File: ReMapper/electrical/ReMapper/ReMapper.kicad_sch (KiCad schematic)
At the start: 7 parts, among them SW1 PU Button, U1 ESP32-S3-WROOM-1-N8R8, U2 SC0914_13_

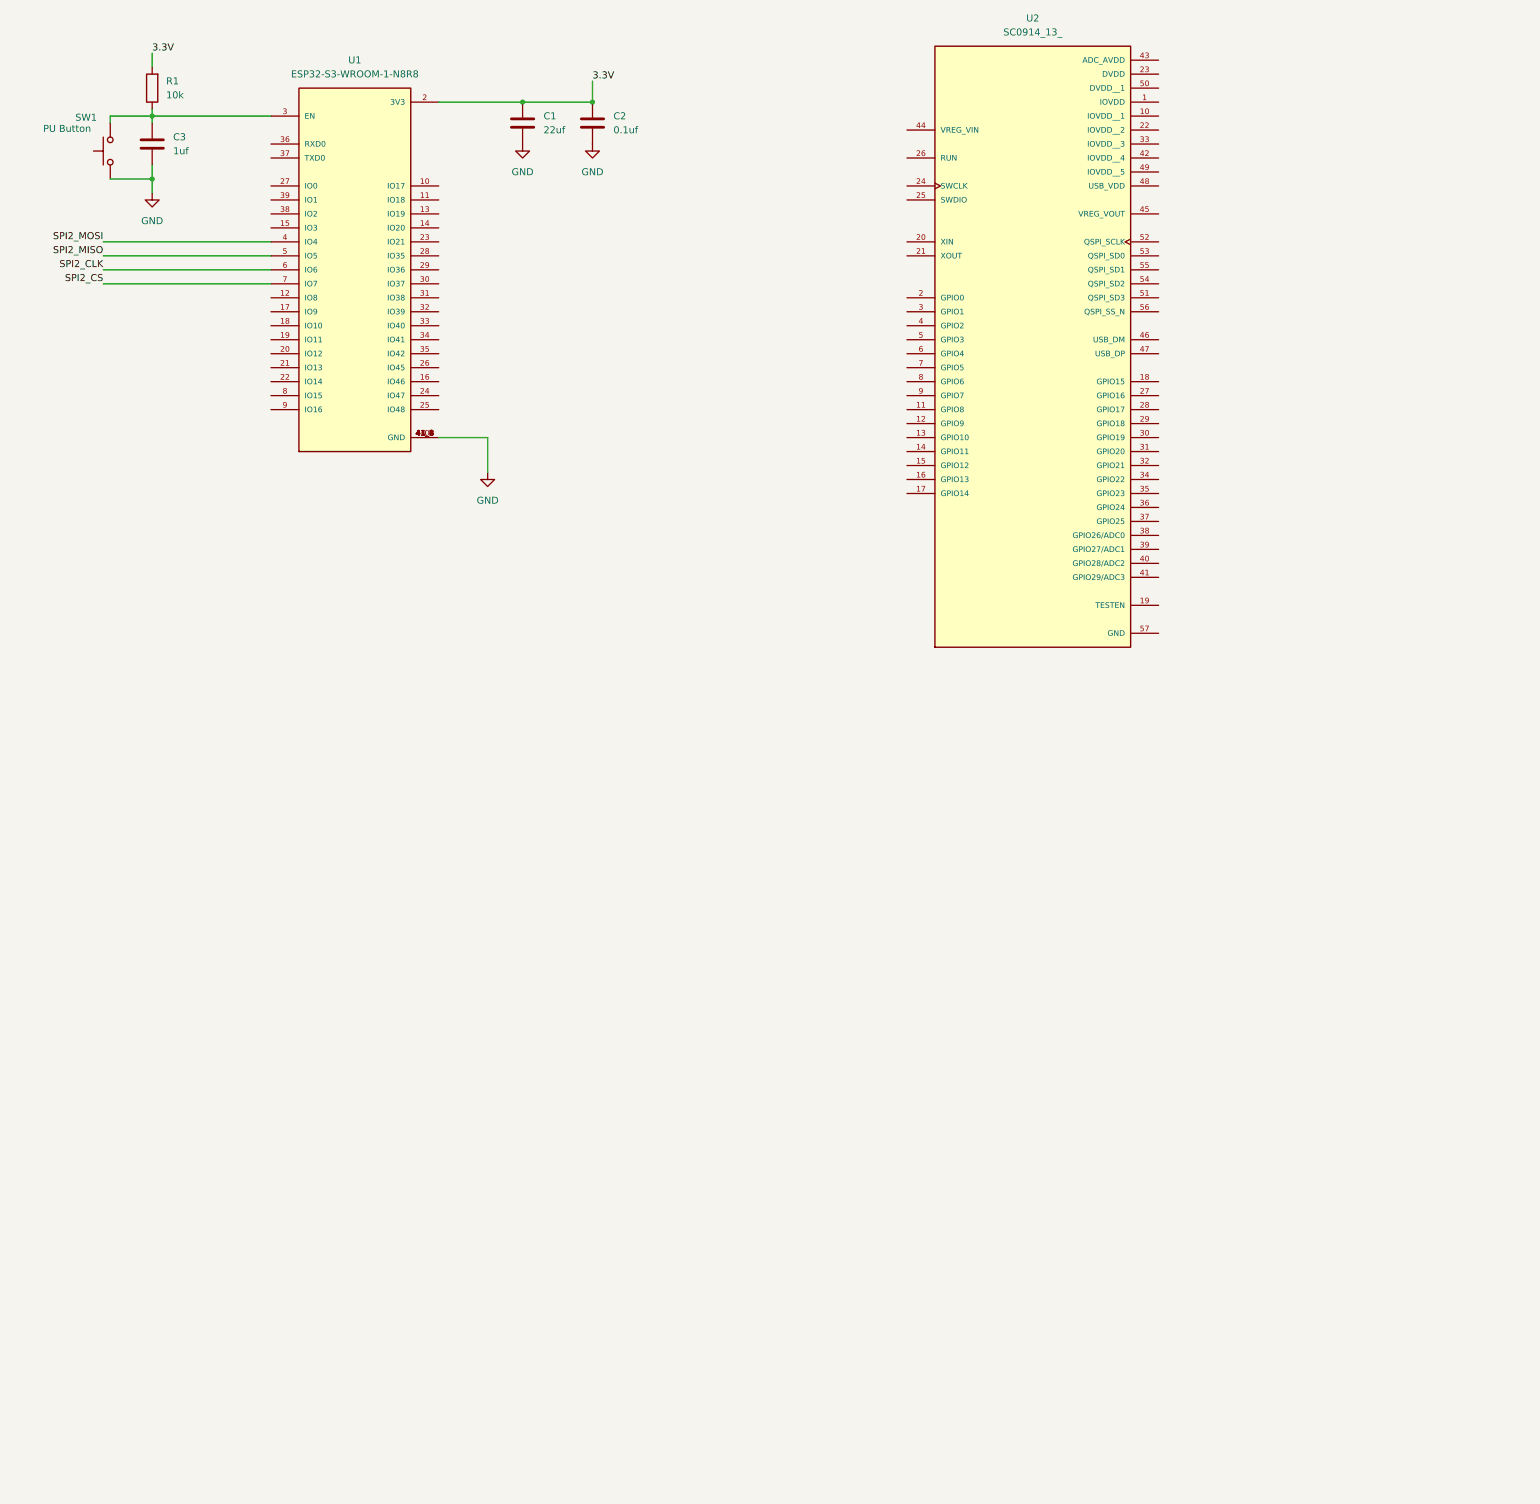
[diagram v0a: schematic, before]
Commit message: more work on schematic
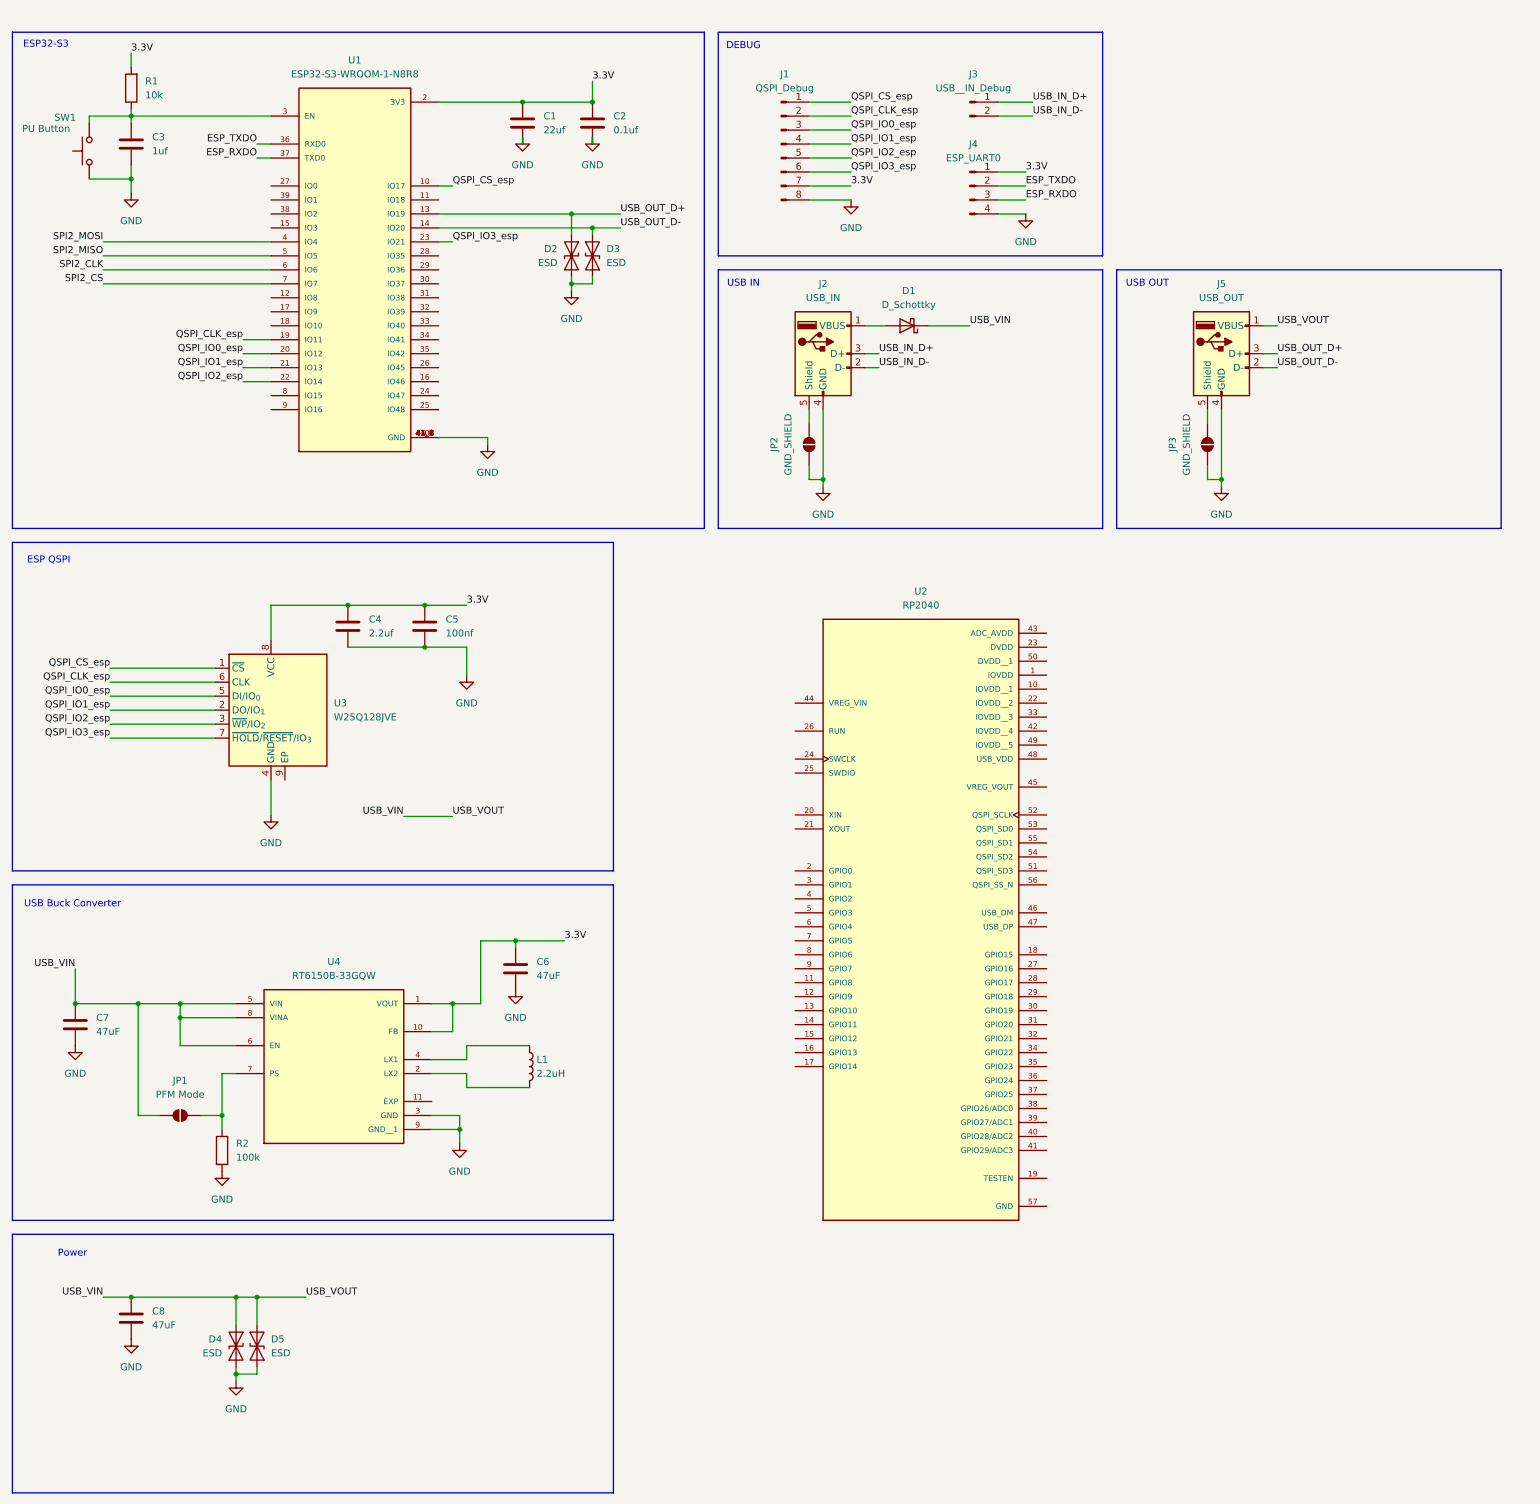
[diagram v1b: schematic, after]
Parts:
- added C4: 2.2uf, symbol Device:C
- added C5: 100nf, symbol Device:C
- added C6, C7, C8: 47uF, symbol Device:C
- added D1: D_Schottky, symbol Device:D_Schottky
- added D2, D3, D4, D5: ESD, Diode_SMD:D_SOD-523, symbol Diode:ESD9B5.0ST5G
- added J1: QSPI_Debug, Connector_PinHeader_1.00mm:PinHeader_1x08_P1.00mm_Vertical, symbol Connector:Conn_01x08_Pin
- added J2: USB_IN, footprints:USBA_Female, symbol Connector:USB_A
- added J3: USB__IN_Debug, Connector_PinHeader_1.00mm:PinHeader_1x02_P1.00mm_Vertical, symbol Connector:Conn_01x02_Pin
- added J4: ESP_UART0, Connector_PinHeader_1.00mm:PinHeader_1x04_P1.00mm_Vertical, symbol Connector:Conn_01x04_Pin
- added J5: USB_OUT, footprints:USBA_Female, symbol Connector:USB_A
- added JP1: PFM Mode, Jumper:SolderJumper-2_P1.3mm_Open_Pad1.0x1.5mm, symbol Jumper:SolderJumper_2_Open
- added JP2, JP3: GND_SHIELD, Jumper:SolderJumper-2_P1.3mm_Open_Pad1.0x1.5mm, symbol Jumper:SolderJumper_2_Open
- added L1: 2.2uH, symbol Device:L
- added R2: 100k, symbol Device:R
- added U3: W25Q128JVE, Package_SON:WSON-8-1EP_8x6mm_P1.27mm_EP3.4x4.3mm, symbol Memory_Flash:W25Q128JVE
- added U4: RT6150B-33GQW, footprints:RT6150B-33GQW, symbol RT6150B-33GQW:RT6150B-33GQW
- U2: value SC0914_13_ -> RP2040
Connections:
- net 3.3V: now also C4.1, C5.1, C6.1, J1.7 (Pin_7), J4.1 (Pin_1), U3.8 (VCC), U4.1 (VOUT), U4.10 (FB)
- net GND: now also C4.2, C5.2, C6.2, C7.2, C8.2, D2.2 (A2), D3.1 (A1), D4.2 (A2), D5.1 (A1), J1.8 (Pin_8), J2.4 (GND), J4.4 (Pin_4), J5.4 (GND), JP2.2 (B), JP3.2 (B), R2.2, U3.4 (GND), U4.3 (GND), U4.9 (GND__1)
- net QSPI_CS_esp: now reaches U1.10 (IO17)
- net QSPI_CS_esp: now also J1.1 (Pin_1), U3.1 (~{CS})
- net USB_OUT_D+: now reaches U1.13 (IO19)
- net USB_OUT_D+: now also D2.1 (A1), J5.3 (D+)
- net USB_OUT_D-: now reaches U1.14 (IO20)
- net USB_OUT_D-: now also D3.2 (A2), J5.2 (D-)
- net QSPI_CLK_esp: now reaches U1.19 (IO11)
- net QSPI_CLK_esp: now also J1.2 (Pin_2), U3.6 (CLK)
- net QSPI_IO0_esp: now reaches U1.20 (IO12)
- net QSPI_IO0_esp: now also J1.3 (Pin_3), U3.5 (DI/IO_{0})
- net QSPI_IO1_esp: now reaches U1.21 (IO13)
- net QSPI_IO1_esp: now also J1.4 (Pin_4), U3.2 (DO/IO_{1})
- net QSPI_IO2_esp: now reaches U1.22 (IO14)
- net QSPI_IO2_esp: now also J1.5 (Pin_5), U3.3 (~{WP}/IO_{2})
- net QSPI_IO3_esp: now reaches U1.23 (IO21)
- net QSPI_IO3_esp: now also J1.6 (Pin_6), U3.7 (~{HOLD}/~{RESET}/IO_{3})
- net ESP_TXDO: now reaches U1.36 (RXD0)
- net ESP_TXDO: now also J4.2 (Pin_2)
- net ESP_RXDO: now reaches U1.37 (TXD0)
- net ESP_RXDO: now also J4.3 (Pin_3)
- new net: J5.5 (Shield), JP3.1 (A)
- new net: J2.5 (Shield), JP2.1 (A)
- new net: JP1.1 (A), R2.1, U4.7 (PS)
- new net: D1.2 (A), J2.1 (VBUS)
- new net: L1.1, U4.4 (LX1)
- new net: L1.2, U4.2 (LX2)
- new net USB_IN_D+: J2.3 (D+), J3.1 (Pin_1)
- new net USB_IN_D-: J2.2 (D-), J3.2 (Pin_2)
- new net USB_VIN: C7.1, C8.1, D1.1 (K), D4.1 (A1), D5.2 (A2), J5.1 (VBUS), JP1.2 (B), U4.5 (VIN), U4.6 (EN), U4.8 (VINA)
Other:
- note added: "DEBUG"
- note added: "ESP QSPI"
- note added: "ESP32-S3"
- note added: "Power"
- note added: "USB Buck Converter"
- note added: "USB IN"
- note added: "USB OUT"
- moved on the sheet: C3, R1, SW1, U2

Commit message: first draft schematic
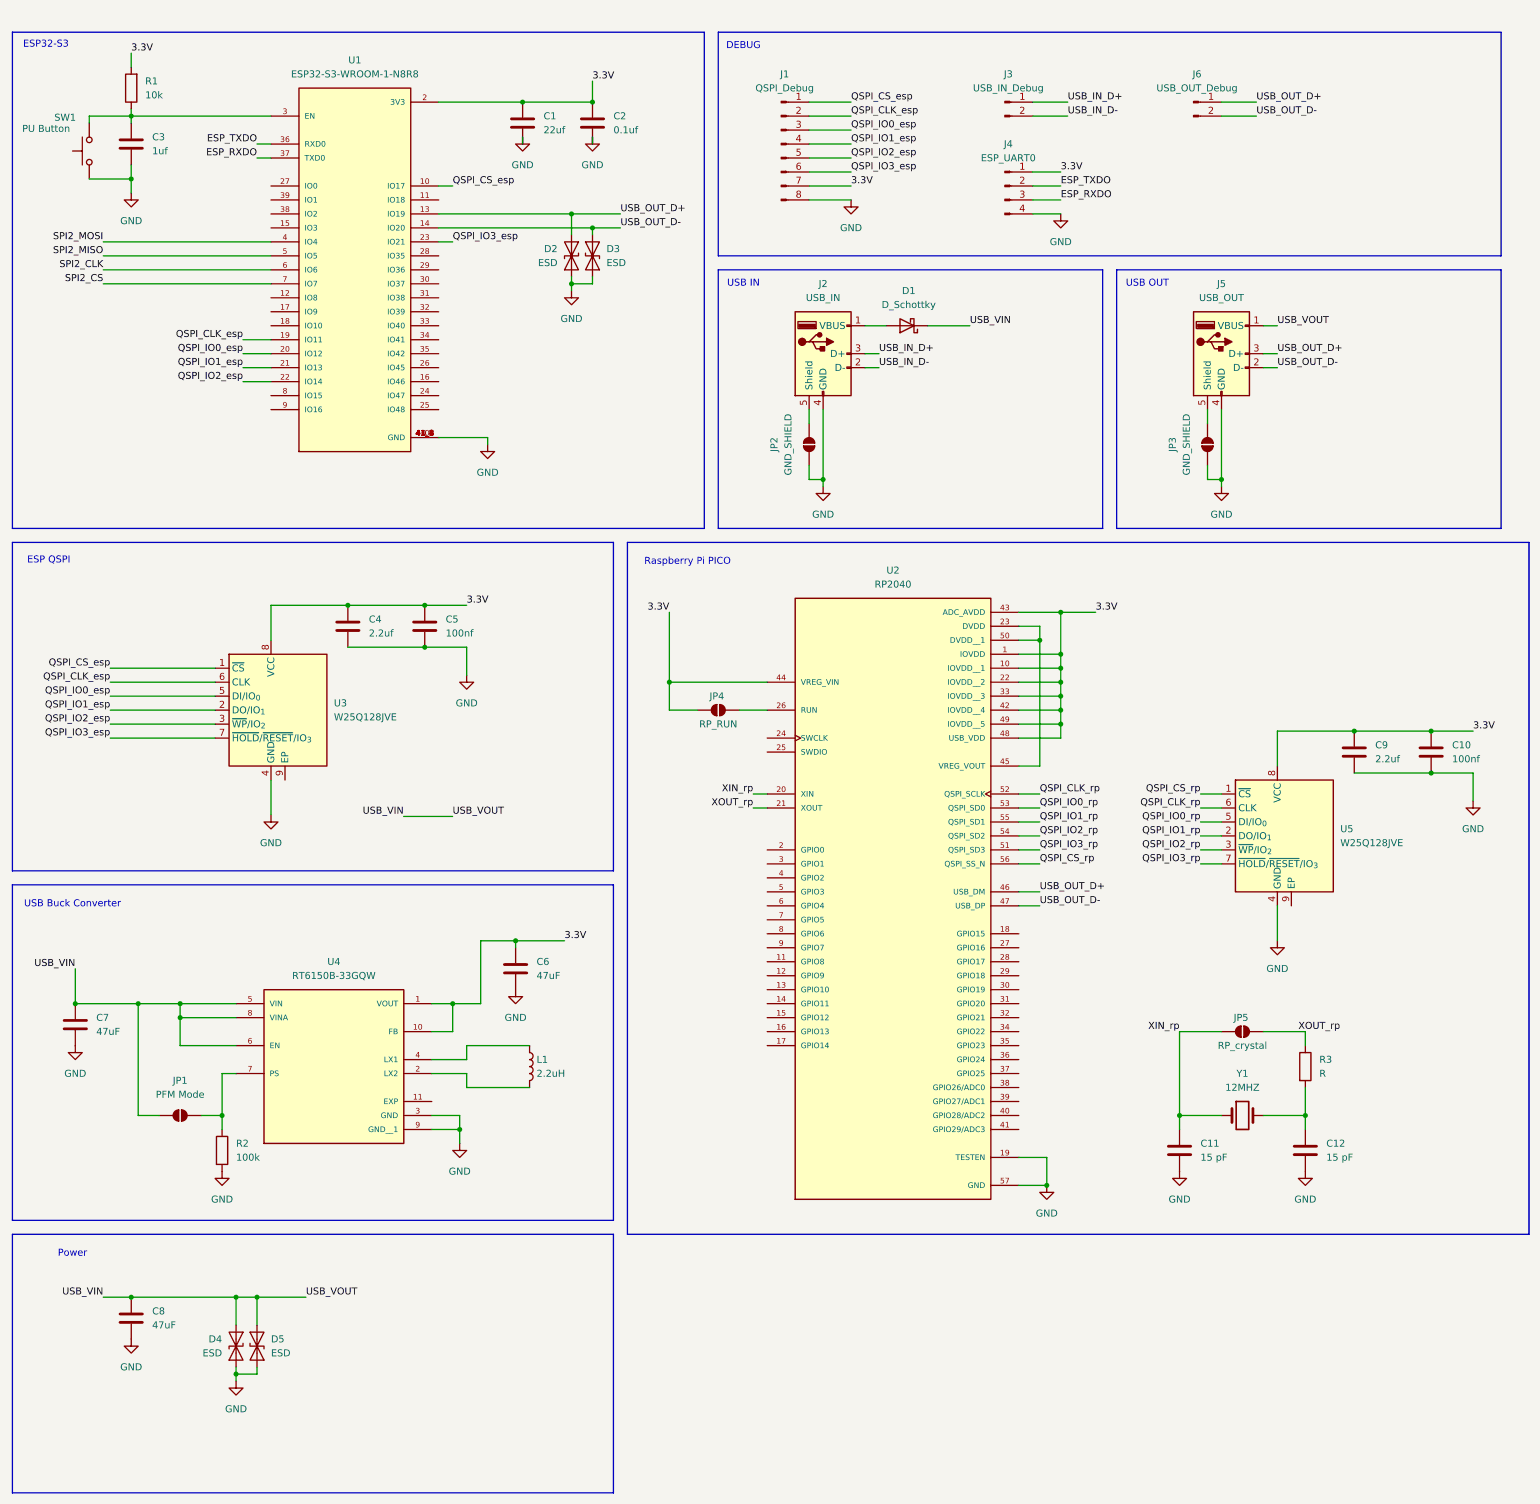
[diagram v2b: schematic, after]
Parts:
- added C10: 100nf, symbol Device:C
- added C11, C12: 15 pF, symbol Device:C
- added C9: 2.2uf, symbol Device:C
- added J6: USB_OUT_Debug, Connector_PinHeader_1.00mm:PinHeader_1x02_P1.00mm_Vertical, symbol Connector:Conn_01x02_Pin
- added JP4: RP_RUN, Jumper:SolderJumper-2_P1.3mm_Open_Pad1.0x1.5mm, symbol Jumper:SolderJumper_2_Open
- added JP5: RP_crystal, Jumper:SolderJumper-2_P1.3mm_Open_Pad1.0x1.5mm, symbol Jumper:SolderJumper_2_Open
- added R3: R, symbol Device:R
- added U5: W25Q128JVE, Package_SON:WSON-8-1EP_8x6mm_P1.27mm_EP3.4x4.3mm, symbol Memory_Flash:W25Q128JVE
- added Y1: 12MHZ, Crystal:Crystal_HC49-4H_Vertical, symbol Device:Crystal
- J3: value USB__IN_Debug -> USB_IN_Debug
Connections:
- net 3.3V: now also U2.1 (IOVDD), U2.10 (IOVDD__1), U2.22 (IOVDD__2), U2.33 (IOVDD__3), U2.42 (IOVDD__4), U2.43 (ADC_AVDD), U2.44 (VREG_VIN), U2.48 (USB_VDD), U2.49 (IOVDD__5), C10.1, C9.1, JP4.1 (A), U5.8 (VCC)
- net GND: now also U2.19 (TESTEN), U2.57 (GND), C10.2, C11.2, C12.2, C9.2, U5.4 (GND)
- net USB_OUT_D+: now also U2.46 (USB_DM), J6.1 (Pin_1)
- net USB_OUT_D-: now also U2.47 (USB_DP), J6.2 (Pin_2)
- net XIN_rp: now reaches U2.20 (XIN)
- net XIN_rp: now also C11.1, JP5.1 (A), Y1.1
- net XOUT_rp: now reaches U2.21 (XOUT)
- net XOUT_rp: now also JP5.2 (B), R3.1
- net at U2.23 (DVDD): now also U2.45 (VREG_VOUT), U2.50 (DVDD__1)
- net at U2.26 (RUN): now also JP4.2 (B)
- net QSPI_IO3_rp: now reaches U2.51 (QSPI_SD3)
- net QSPI_IO3_rp: now also U5.7 (~{HOLD}/~{RESET}/IO_{3})
- net QSPI_CLK_rp: now reaches U2.52 (QSPI_SCLK)
- net QSPI_CLK_rp: now also U5.6 (CLK)
- net QSPI_IO0_rp: now reaches U2.53 (QSPI_SD0)
- net QSPI_IO0_rp: now also U5.5 (DI/IO_{0})
- net QSPI_IO2_rp: now reaches U2.54 (QSPI_SD2)
- net QSPI_IO2_rp: now also U5.3 (~{WP}/IO_{2})
- net QSPI_IO1_rp: now reaches U2.55 (QSPI_SD1)
- net QSPI_IO1_rp: now also U5.2 (DO/IO_{1})
- net QSPI_CS_rp: now reaches U2.56 (QSPI_SS_N)
- net QSPI_CS_rp: now also U5.1 (~{CS})
- new net: C12.1, R3.2, Y1.2
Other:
- note added: "Raspberry Pi PICO"
- moved on the sheet: J3, J4, U2
